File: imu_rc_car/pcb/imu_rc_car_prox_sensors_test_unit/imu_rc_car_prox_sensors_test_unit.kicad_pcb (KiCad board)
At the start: 2 copper layers, 33.4 x 29.2 mm, 10 parts, among them J1 Conn_01x04_Socket

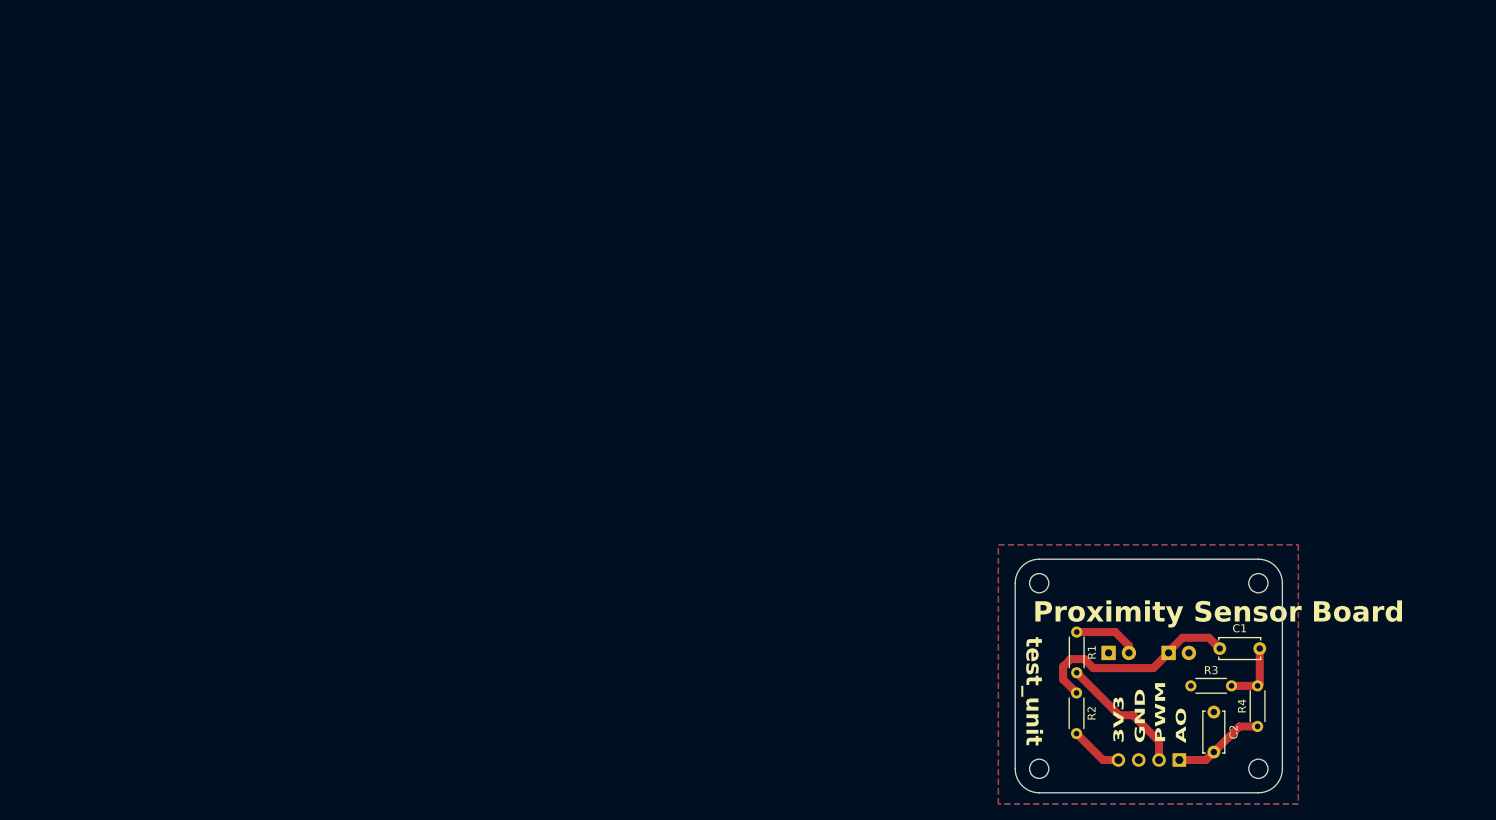
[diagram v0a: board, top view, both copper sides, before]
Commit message: commit #25
added library for mouse-bites
minor changes in prox sensors board
added necessary changes for test unit to print
minor changes in hand unit
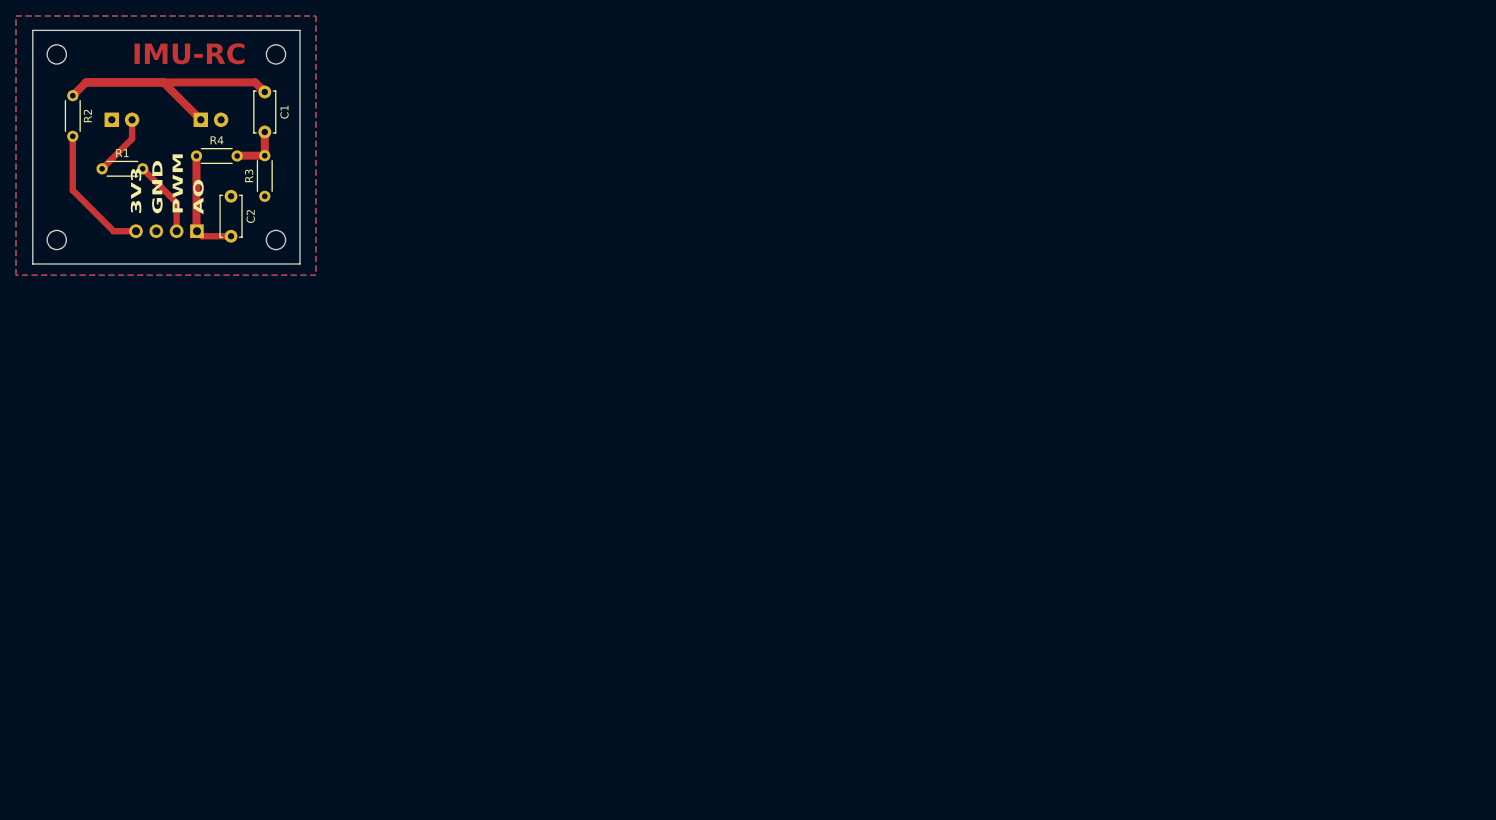
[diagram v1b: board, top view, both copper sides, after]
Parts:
- removed G***: LOGO, LOGO
- moved R4 150.6 mm to (32.7, 27.9), turned to 0 degrees
- moved R2 146.0 mm to (17.2, 20.4)
- moved Emissor 141.3 mm to (22.1, 23.4)
- moved J1 139.5 mm to (32.7, 37.3)
- moved C2 138.7 mm to (37.0, 32.9)
- moved C1 138.2 mm to (41.2, 19.9), turned to -90 degrees
- moved Recetor 138.1 mm to (33.2, 23.4)
- moved R1 134.9 mm to (20.9, 29.5), turned to 0 degrees
- moved R3 130.9 mm to (41.2, 32.9), turned to 90 degrees
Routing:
- net Net-(Recetor1-K): track 26.7 -> 41.5 mm
- net +3V3: track 6.60 -> 16.8 mm
- net PWM: track 16.2 -> 9.56 mm
- net AO: track 11.5 -> 13.9 mm
- net Net-(C1-Pad2): track 8.03 -> 6.44 mm
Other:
- outline, holes or cut-outs redrawn
- board text added: "IMU-RC"
- board text removed: "ESTG-IPL"
- board text removed: "Proximity Sensor Board"
- board text removed: "test_unit"
